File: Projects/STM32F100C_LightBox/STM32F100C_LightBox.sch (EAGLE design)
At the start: 29 parts, among them CN1 1X4-3.5MM, CN2 1X4-3.5MM, CN3 1X4-3.5MM, CN4 1X4-3.5MM

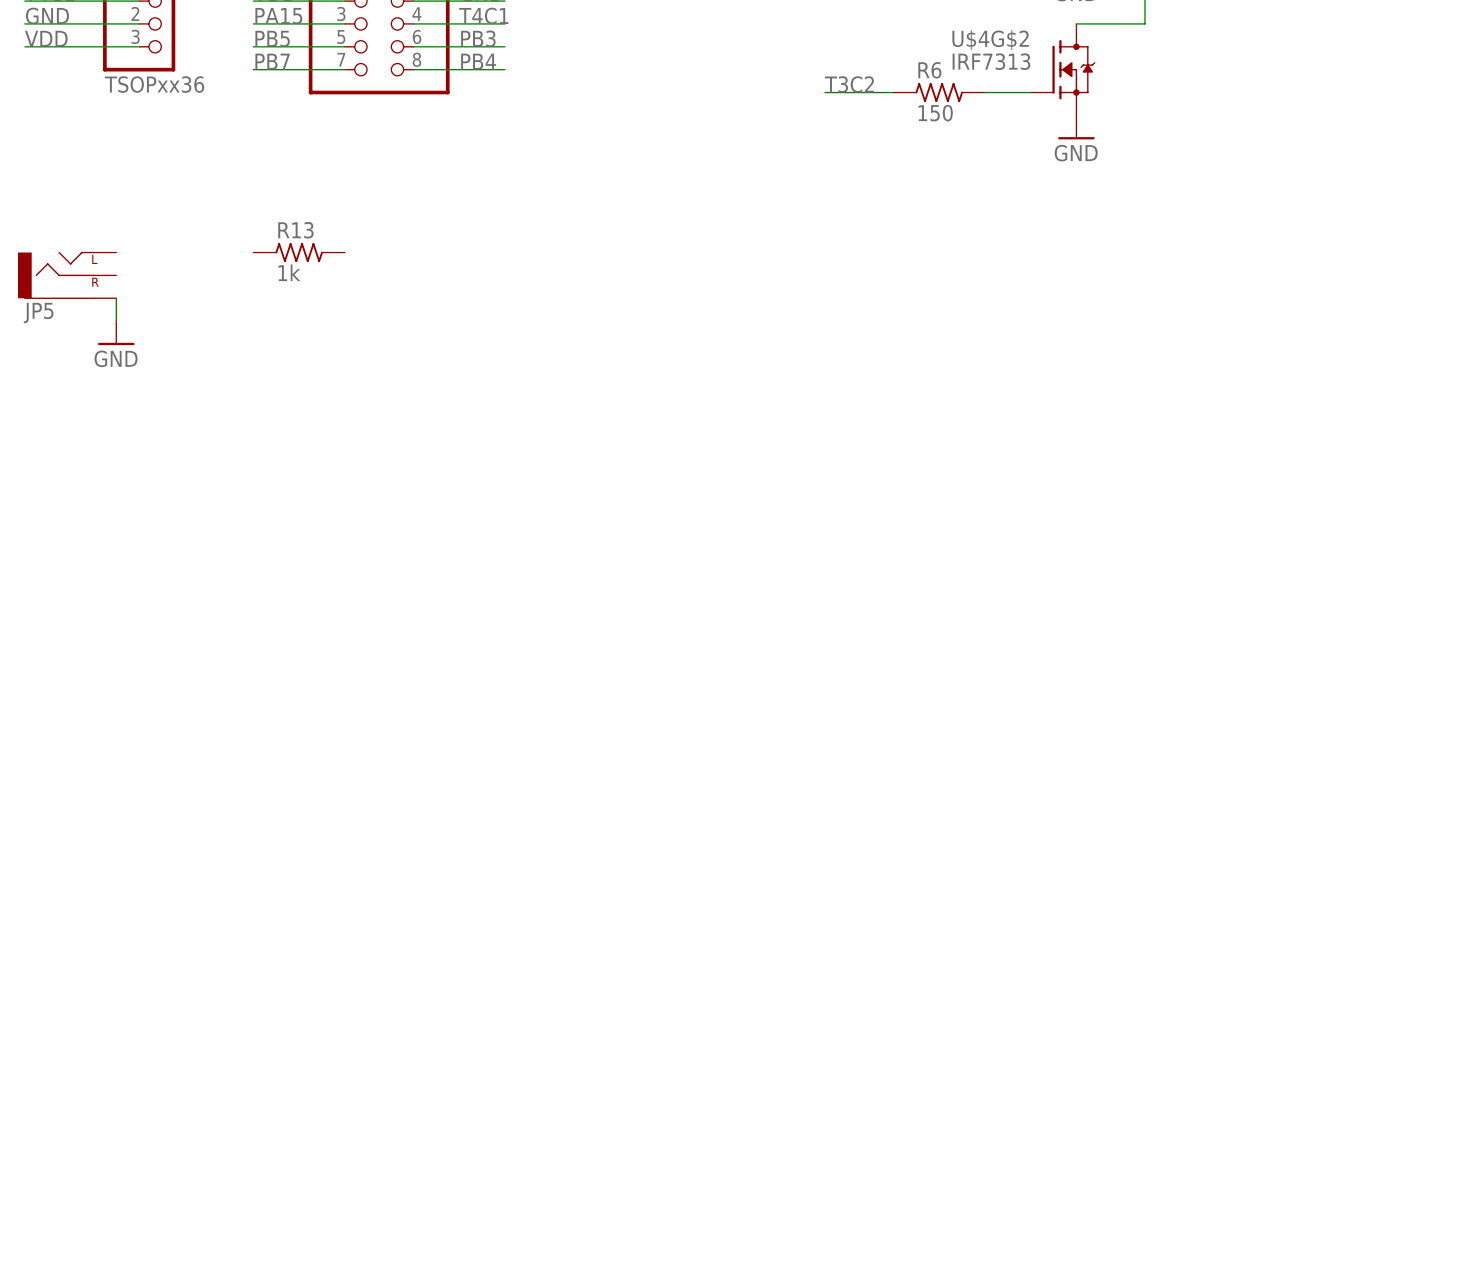
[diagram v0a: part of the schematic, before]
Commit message: LB Audio in...
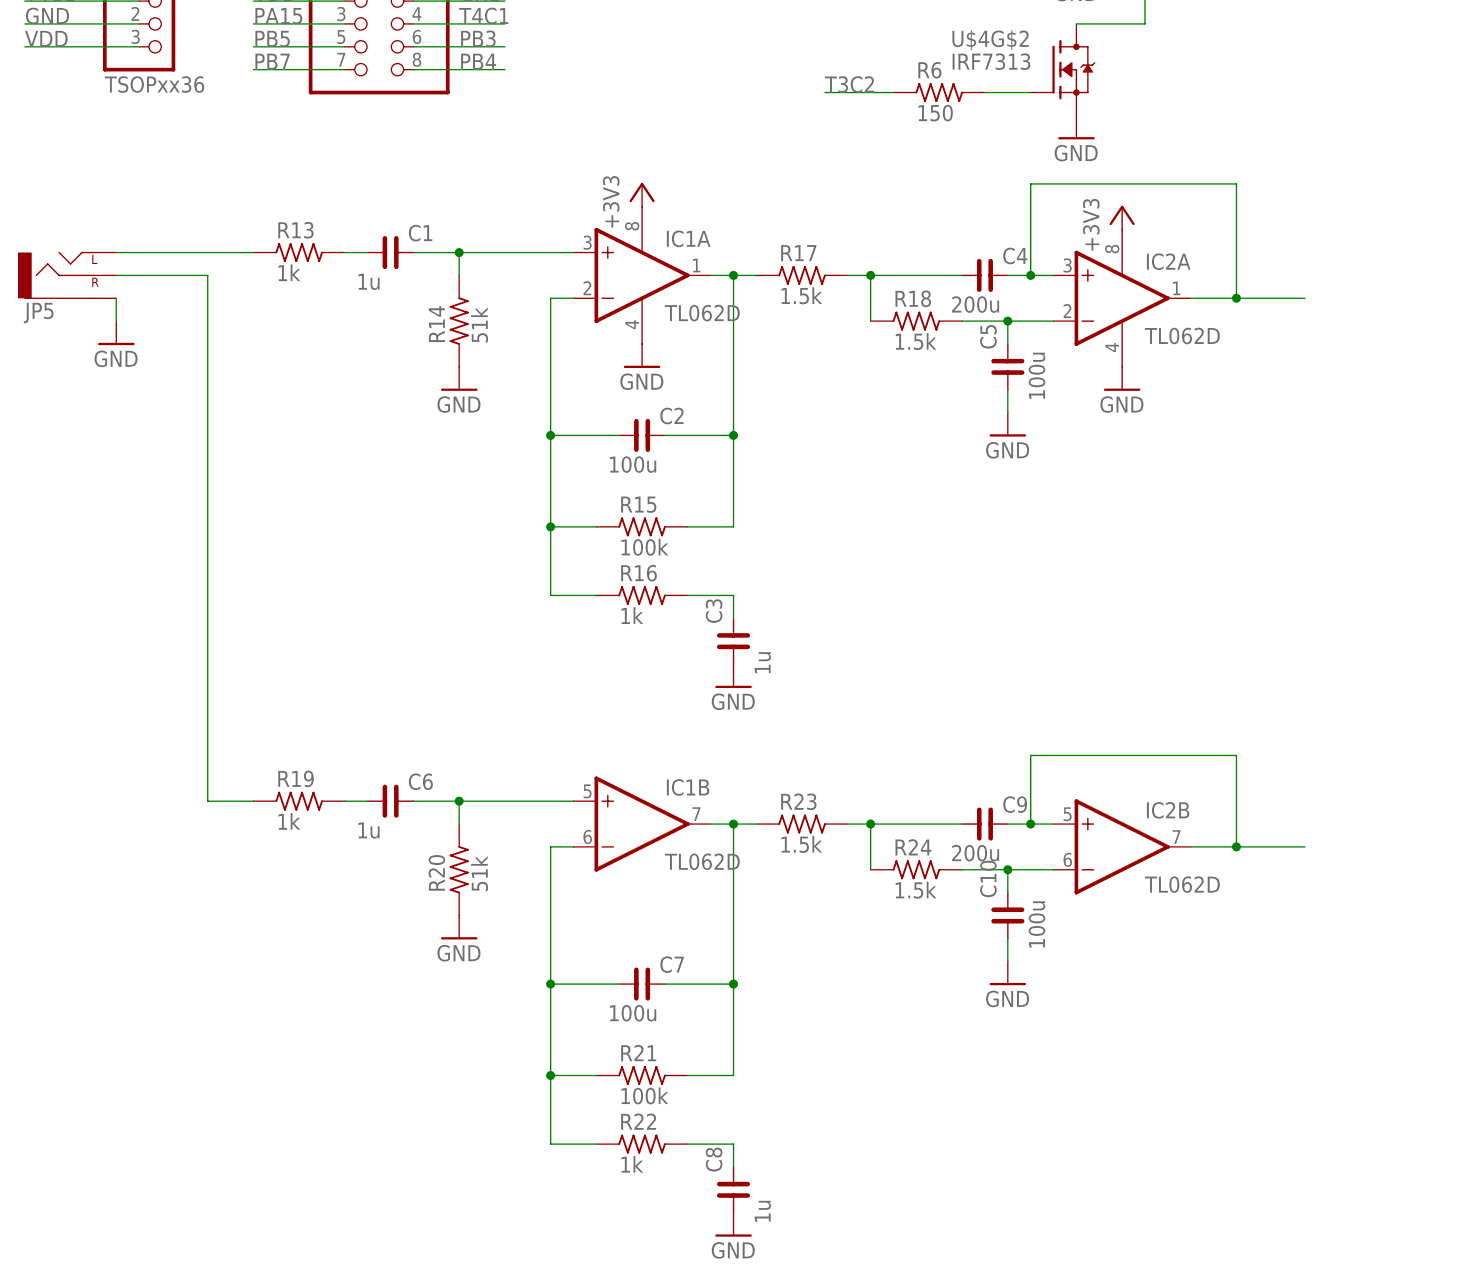
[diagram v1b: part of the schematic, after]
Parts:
- added C1, C3, C6, C8: 1u, rc-master-smd:C_0603
- added C10, C2, C5, C7: 100u, rc-master-smd:C_0603
- added C4, C9: 200u, rc-master-smd:C_0603
- added IC1, IC2: TL062D, linear:TL062D
- added R14, R20: 51k, rc-master-smd:R_1206
- added R15, R21: 100k, rc-master-smd:R_1206
- added R16, R19, R22: 1k, rc-master-smd:R_1206
- added R17, R18, R23, R24: 1.5k, rc-master-smd:R_1206
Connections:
- new net +3V3: IC1P.V+, IC2P.V+
- new net N$25: JP5.LEFT, R13.1
- new net N$26: C1.1, R13.2
- new net N$27: C1.2, IC1A.+IN, R14.2
- new net N$28: C2.1, IC1A.-IN, R15.1, R16.1
- new net N$29: C2.2, IC1A.OUT, R15.2, R17.1
- new net N$30: C3.2, R16.2
- new net N$31: JP5.RIGHT, R19.1
- new net N$32: C5.2, IC2A.-IN, R18.2
- new net N$33: C4.1, R17.2, R18.1
- new net N$34: C4.2, IC2A.+IN, IC2A.OUT
- new net N$35: C6.1, R19.2
- new net N$36: C6.2, IC1B.+IN, R20.2
- new net N$37: C7.1, IC1B.-IN, R21.1, R22.1
- new net N$38: C7.2, IC1B.OUT, R21.2, R23.1
- new net N$39: C8.2, R22.2
- new net N$40: C9.1, R23.2, R24.1
- new net N$41: C10.2, IC2B.-IN, R24.2
- new net N$42: C9.2, IC2B.+IN, IC2B.OUT
- net GND: now also C10.1, C3.1, C5.1, C8.1, IC1P.V-, IC2P.V-, R14.1, R20.1
